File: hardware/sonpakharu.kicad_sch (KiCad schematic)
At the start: 11 parts, among them IC1 ESP32-S3-WROOM-1U-N4, J1 USB_OTG, J2 UART, J3 Boot option, SW1 Reset

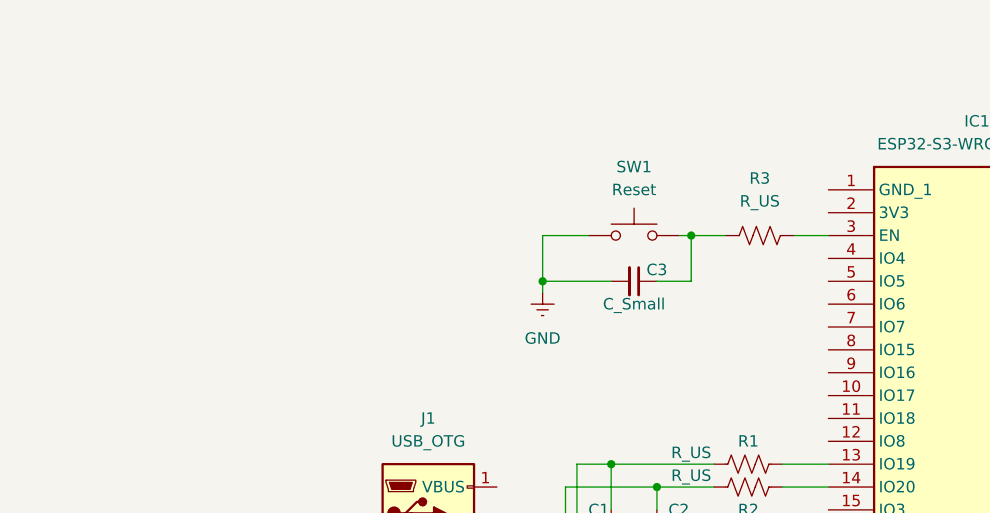
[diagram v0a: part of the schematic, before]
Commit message: minor changes
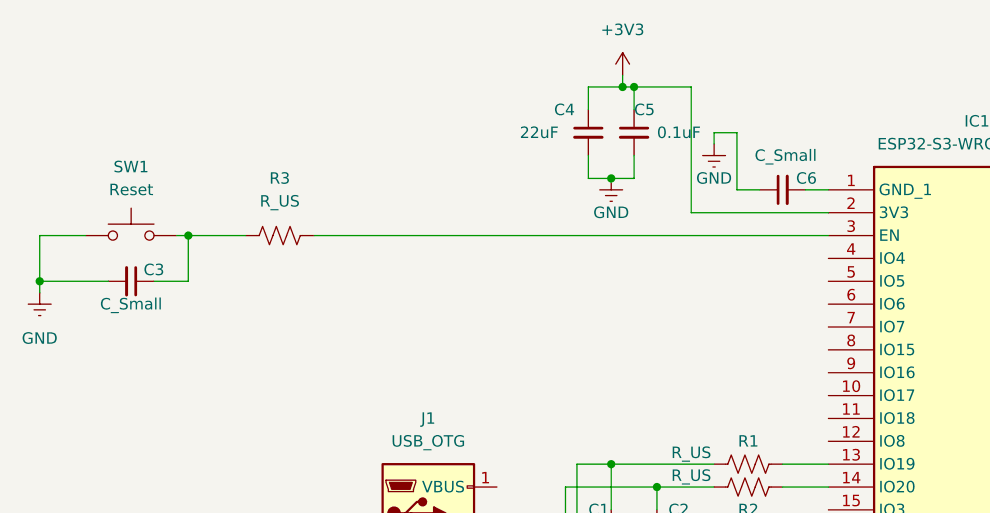
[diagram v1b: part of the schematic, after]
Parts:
- added C4: 22uF, symbol Device:C_Small
- added C5: 0.1uF, symbol Device:C_Small
- added C6: C_Small, symbol Device:C_Small
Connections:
- net GND: now also C4.2, C5.2, C6.1
- net at IC1.1 (GND_1): now also C6.2
- net +3V3: now reaches IC1.2 (3V3)
- net +3V3: now also C4.1, C5.1
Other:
- moved on the sheet: C3, R3, SW1
